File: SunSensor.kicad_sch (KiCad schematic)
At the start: 6 parts, among them U1 AD7291BCPZ

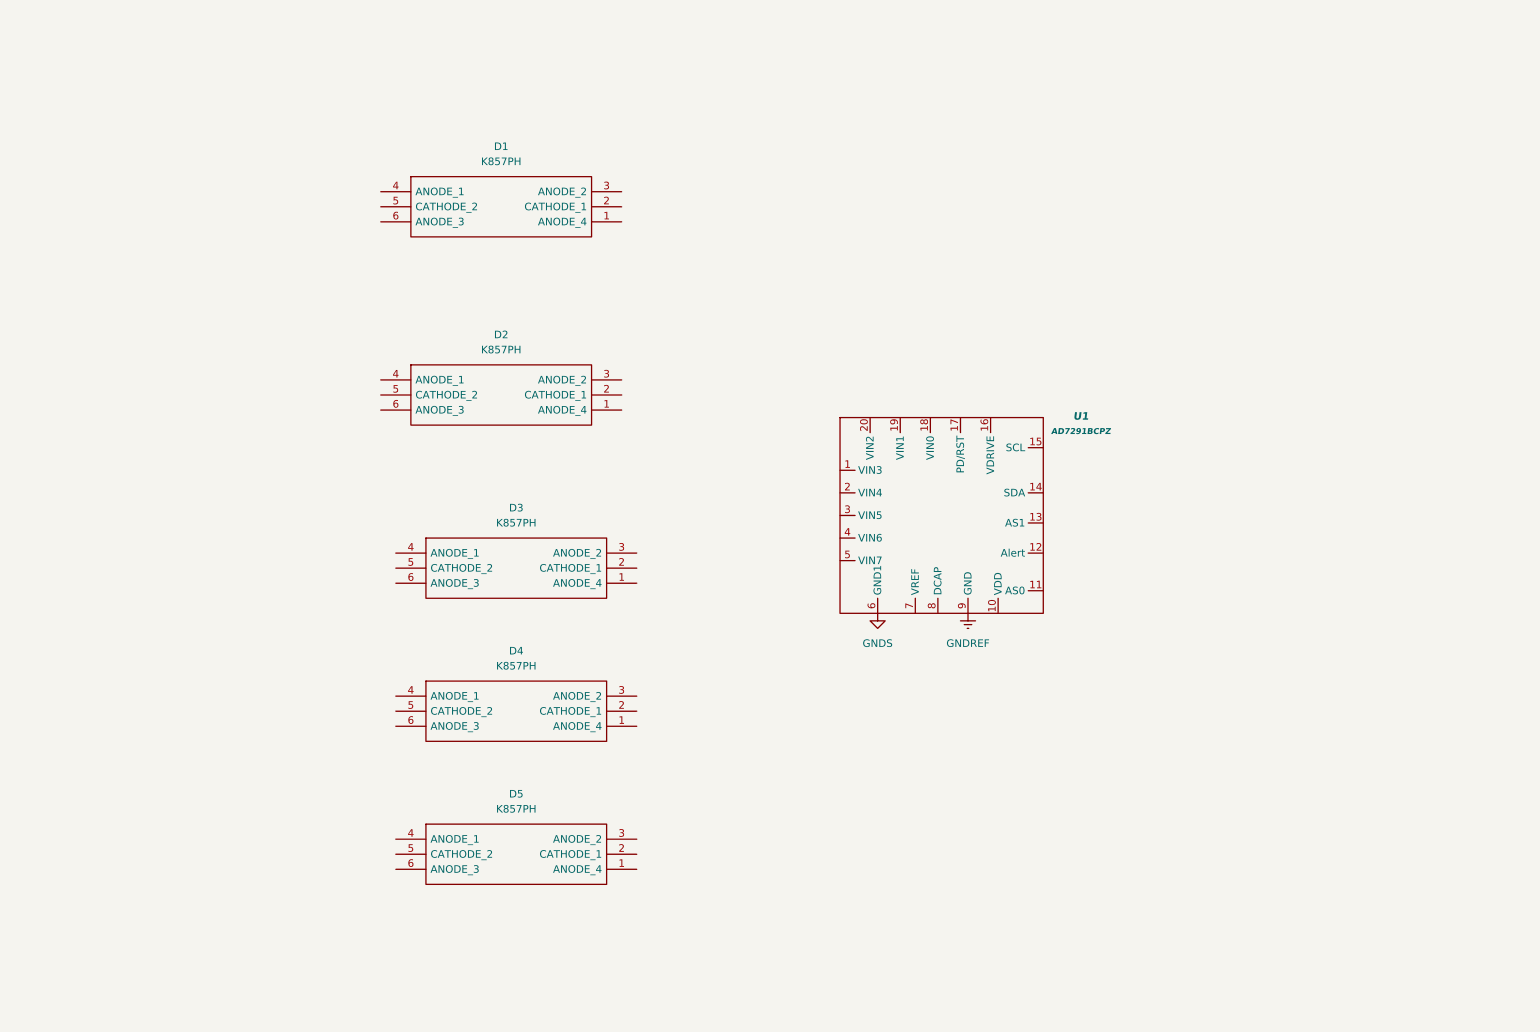
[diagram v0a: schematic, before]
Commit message: Finished schematic and finalized parts
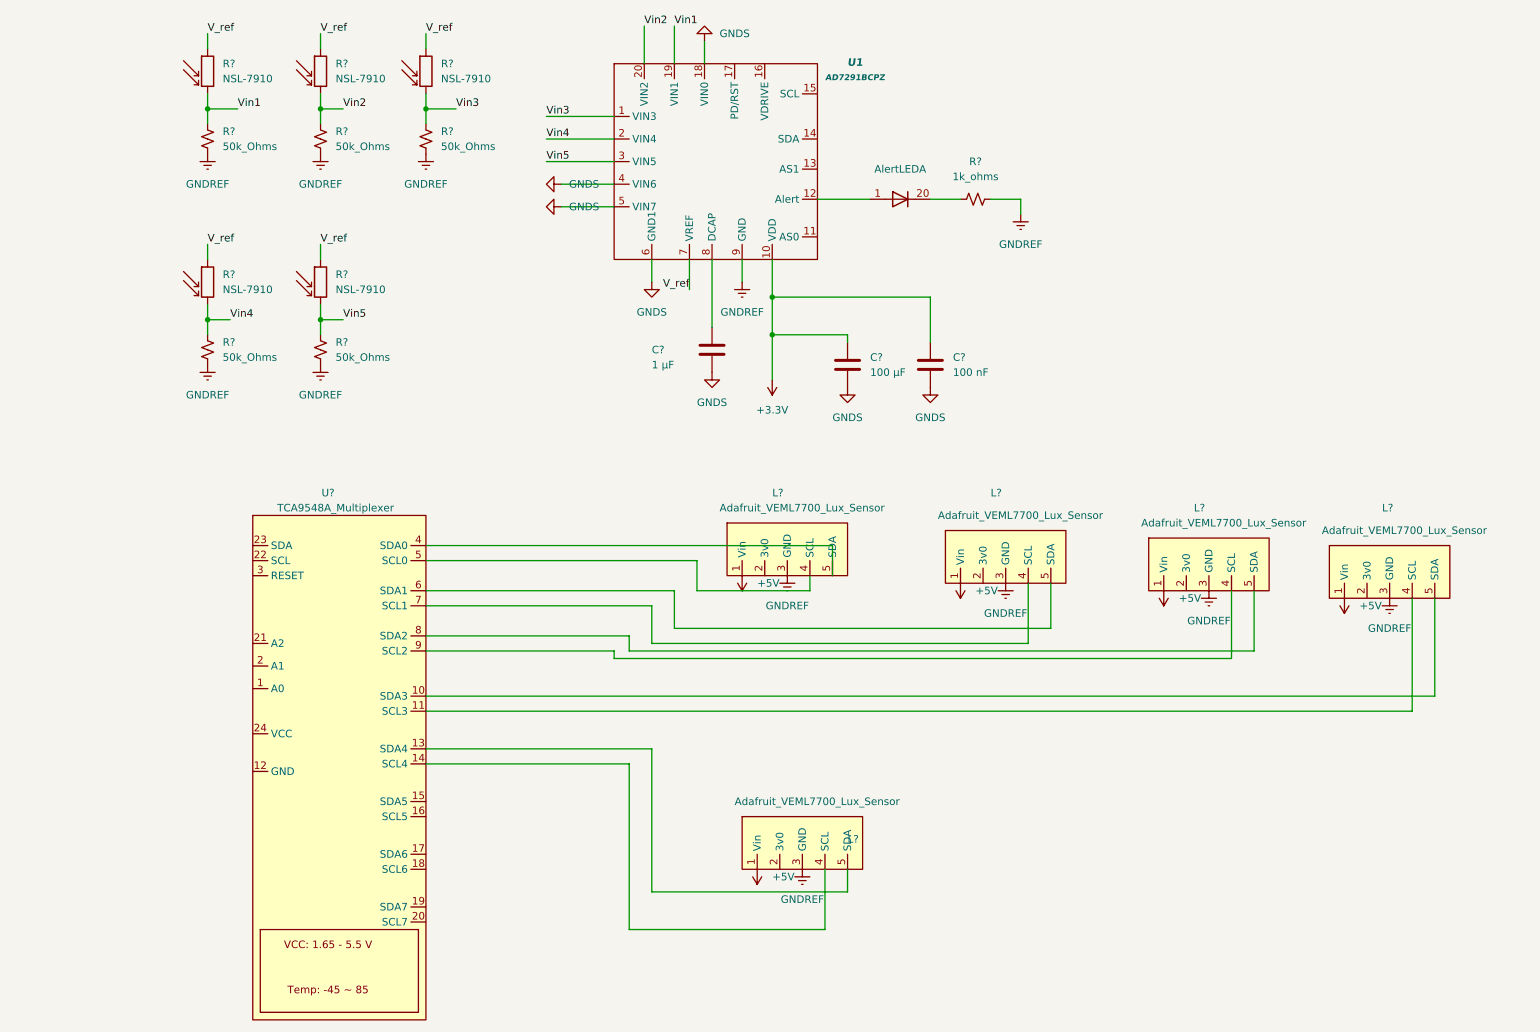
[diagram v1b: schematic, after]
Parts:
- removed D1, D2, D3, D4, D5: K857PH, K857PH, symbol Diode:K857PH
- added AlertLED: (no value), Display:HDSP-4836, symbol LED:HDSP-4836
- added C?: 1 µF, symbol Device:C
- added C?: 100 µF, symbol Device:C
- added C?: 100 nF, symbol Device:C
- added L? (x5): Adafruit_VEML7700_Lux_Sensor, symbol Sensor_Optical:Adafruit_VEML7700_Lux_Sensor
- added R? (x5): NSL-7910, symbol Device:R_Photo
- added R? (x5): 50k_Ohms, symbol Device:50k_Ohms
- added R?: 1k_ohms, symbol Device:50k_Ohms
- added U?: TCA9548A_Multiplexer, symbol Analog_Switch:TCA9548A_Multiplexer
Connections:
- net GNDREF: now also L?.3 (GND), L?.3 (GND), L?.3 (GND), L?.3 (GND), L?.3 (GND), R?.2, R?.2, R?.2, R?.2, R?.2, R?.2
- net GNDS: now also U1.18 (VIN0), U1.4 (VIN6), U1.5 (VIN7), C?.2, C?.2, C?.2
- net Vin3: now reaches U1.1 (VIN3)
- net Vin3: now also R?.1, R?.2
- net +3V3: now reaches U1.10 (VDD)
- net +3V3: now also C?.1, C?.1
- net at U1.12 (Alert): now also AlertLED.1 (A)
- net Vin1: now reaches U1.19 (VIN1)
- net Vin1: now also R?.1, R?.2
- net Vin4: now reaches U1.2 (VIN4)
- net Vin4: now also R?.1, R?.2
- net Vin2: now reaches U1.20 (VIN2)
- net Vin2: now also R?.1, R?.2
- net Vin5: now reaches U1.3 (VIN5)
- net Vin5: now also R?.1, R?.2
- net V_ref: now reaches U1.7 (VREF)
- net V_ref: now also R?.1, R?.1, R?.1, R?.1, R?.1
- net at U1.8 (DCAP): now also C?.1
- new net: L?.4 (SCL), U?.5 (SCL0)
- new net: L?.5 (SDA), U?.4 (SDA0)
- new net: L?.4 (SCL), U?.11 (SCL3)
- new net: L?.5 (SDA), U?.10 (SDA3)
- new net: L?.4 (SCL), U?.14 (SCL4)
- new net: L?.5 (SDA), U?.13 (SDA4)
- new net: L?.4 (SCL), U?.7 (SCL1)
- new net: L?.5 (SDA), U?.6 (SDA1)
- new net: L?.4 (SCL), U?.9 (SCL2)
- new net: L?.5 (SDA), U?.8 (SDA2)
- new net: AlertLED.20 (K), R?.1
- new net +5V: L?.1 (Vin), L?.1 (Vin), L?.1 (Vin), L?.1 (Vin), L?.1 (Vin)
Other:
- moved on the sheet: U1
